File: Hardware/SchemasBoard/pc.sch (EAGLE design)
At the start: 10 parts

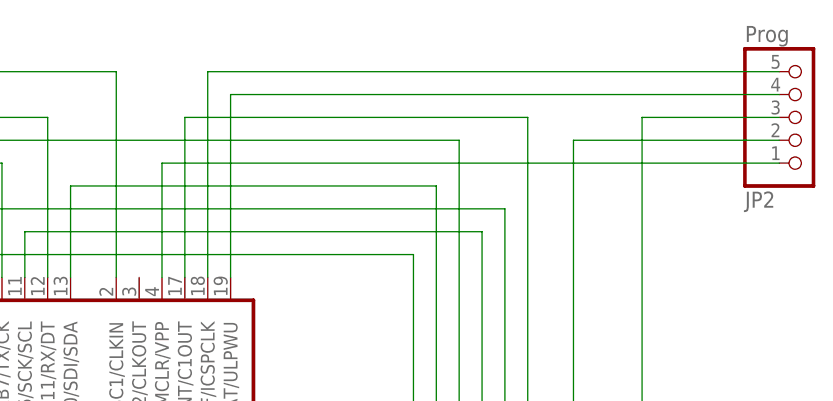
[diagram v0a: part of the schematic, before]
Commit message: aaa
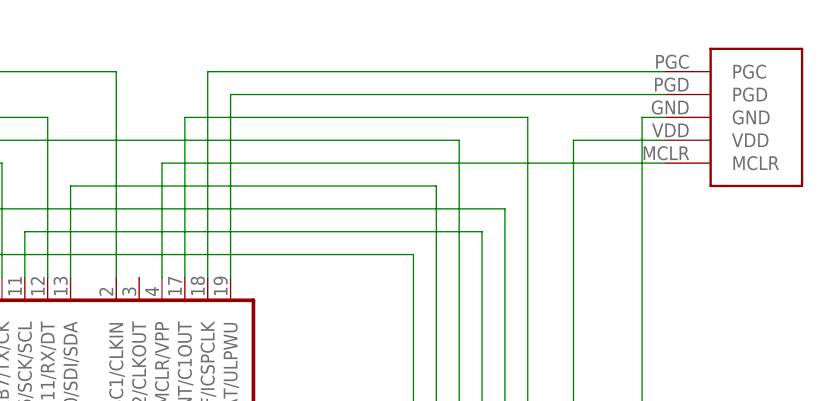
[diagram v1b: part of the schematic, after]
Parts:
- removed JP2: Prog, pinhead:PINHD-1X5
- added U$3: PROGRAMMINGHEADERDIP, rfm70:PROGRAMMINGHEADERDIP
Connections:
- removed net N$19: JP2.5, U$2.RA1/AN1/C12IN0-/VREF/ICSPCLK
- new net N$2: U$2.RA1/AN1/C12IN0-/VREF/ICSPCLK, U$3.PGC
- net GND: now also U$3.GND; no longer JP2.3
- net N$18: now also U$3.PGD; no longer JP2.4
- net N$25: now also U$3.MCLR; no longer JP2.1
- net VDD: now also U$3.VDD; no longer JP2.2
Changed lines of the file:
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@@
 <part name="U$1" library="rfm70" deviceset="RFM70" device=""/>
 <part name="U$2" library="microchip" deviceset="PIC16F690*" device=""/>
-<part name="JP2" library="pinhead" deviceset="PINHD-1X5" device="" value="Prog"/>
 <part name="PAD1" library="wirepad" deviceset="WIREPAD" device="SMD5-1,8"/>
 <part name="PAD2" library="wirepad" deviceset="WIREPAD" device="SMD5-1,8"/>
@@
 <part name="C2" library="resistor" deviceset="CPOL-EU" device="SMCA" value="1uF"/>
 <part name="S2" library="switch-tact" deviceset="DTSM-3" device=""/>
+<part name="U$3" library="rfm70" deviceset="PROGRAMMINGHEADER" device="" technology="DIP"/>
 </parts>
 <sheets>
@@
 <instance part="U$1" gate="G$1" x="170.18" y="45.72" rot="R270"/>
 <instance part="U$2" gate="G$1" x="134.62" y="68.58" rot="R90"/>
-<instance part="JP2" gate="A" x="195.58" y="137.16" rot="MR180"/>
 <instance part="PAD1" gate="G$1" x="38.1" y="83.82"/>
 <instance part="PAD2" gate="G$1" x="38.1" y="78.74"/>
@@
 <instance part="C2" gate="G$1" x="106.68" y="48.26"/>
 <instance part="S2" gate="G$1" x="68.58" y="50.8"/>
+<instance part="U$3" gate="G$1" x="190.5" y="137.16"/>
 </instances>
 <busses>
@@
 <wire x1="172.72" y1="55.88" x2="177.8" y2="55.88" width="0.1524" layer="91"/>
 <wire x1="177.8" y1="55.88" x2="177.8" y2="30.48" width="0.1524" layer="91"/>
-<wire x1="193.04" y1="137.16" x2="177.8" y2="137.16" width="0.1524" layer="91"/>
+<wire x1="180.34" y1="137.16" x2="177.8" y2="137.16" width="0.1524" layer="91"/>
 <wire x1="177.8" y1="137.16" x2="177.8" y2="55.88" width="0.1524" layer="91"/>
 <junction x="177.8" y="55.88"/>
 <junction x="132.08" y="30.48"/>
-<pinref part="JP2" gate="A" pin="3"/>
 <wire x1="40.64" y1="68.58" x2="40.64" y2="30.48" width="0.1524" layer="91"/>
 <pinref part="PAD4" gate="G$1" pin="P"/>
@@
 <wire x1="68.58" y1="30.48" x2="68.58" y2="45.72" width="0.1524" layer="91"/>
 <pinref part="S2" gate="G$1" pin="1"/>
+<pinref part="U$3" gate="G$1" pin="GND"/>
 </segment>
 </net>
@@
 <wire x1="170.18" y1="63.5" x2="170.18" y2="134.62" width="0.1524" layer="91"/>
 <junction x="170.18" y="63.5"/>
-<pinref part="JP2" gate="A" pin="2"/>
-<wire x1="170.18" y1="134.62" x2="193.04" y2="134.62" width="0.1524" layer="91"/>
+<wire x1="170.18" y1="134.62" x2="180.34" y2="134.62" width="0.1524" layer="91"/>
 <wire x1="33.02" y1="83.82" x2="33.02" y2="63.5" width="0.1524" layer="91"/>
 <wire x1="33.02" y1="63.5" x2="83.82" y2="63.5" width="0.1524" layer="91"/>
@@
 <junction x="88.9" y="63.5"/>
 <junction x="106.68" y="63.5"/>
+<pinref part="U$3" gate="G$1" pin="VDD"/>
 </segment>
 </net>
@@
 <pinref part="U$2" gate="G$1" pin="RA0/AN0/C1IN+/ICSPDAT/ULPWU"/>
 <wire x1="132.08" y1="139.7" x2="132.08" y2="119.38" width="0.1524" layer="91"/>
-<pinref part="JP2" gate="A" pin="4"/>
-<wire x1="193.04" y1="139.7" x2="132.08" y2="139.7" width="0.1524" layer="91"/>
-</segment>
-</net>
-<net name="N$19" class="0">
-<segment>
-<pinref part="U$2" gate="G$1" pin="RA1/AN1/C12IN0-/VREF/ICSPCLK"/>
-<wire x1="129.54" y1="142.24" x2="129.54" y2="119.38" width="0.1524" layer="91"/>
-<pinref part="JP2" gate="A" pin="5"/>
-<wire x1="129.54" y1="142.24" x2="193.04" y2="142.24" width="0.1524" layer="91"/>
+<wire x1="180.34" y1="139.7" x2="132.08" y2="139.7" width="0.1524" layer="91"/>
+<pinref part="U$3" gate="G$1" pin="PGD"/>
 </segment>
 </net>
@@
 <pinref part="U$2" gate="G$1" pin="RA3/MCLR/VPP"/>
 <wire x1="124.46" y1="119.38" x2="124.46" y2="132.08" width="0.1524" layer="91"/>
-<pinref part="JP2" gate="A" pin="1"/>
-<wire x1="124.46" y1="132.08" x2="193.04" y2="132.08" width="0.1524" layer="91"/>
+<wire x1="124.46" y1="132.08" x2="180.34" y2="132.08" width="0.1524" layer="91"/>
+<pinref part="U$3" gate="G$1" pin="MCLR"/>
 </segment>
 </net>
@@
 </segment>
 </net>
+<net name="N$2" class="0">
+<segment>
+<pinref part="U$3" gate="G$1" pin="PGC"/>
+<pinref part="U$2" gate="G$1" pin="RA1/AN1/C12IN0-/VREF/ICSPCLK"/>
+<wire x1="180.34" y1="142.24" x2="129.54" y2="142.24" width="0.1524" layer="91"/>
+<wire x1="129.54" y1="142.24" x2="129.54" y2="119.38" width="0.1524" layer="91"/>
+</segment>
+</net>
